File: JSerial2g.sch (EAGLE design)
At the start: 59 parts, among them CN1 USBMOLEX, IC1 FT232RL, Q1 2N3904SOT23, Q2 2N3904SOT23, Q3 BC547, Q4 BC547, X1 RJ45-8X

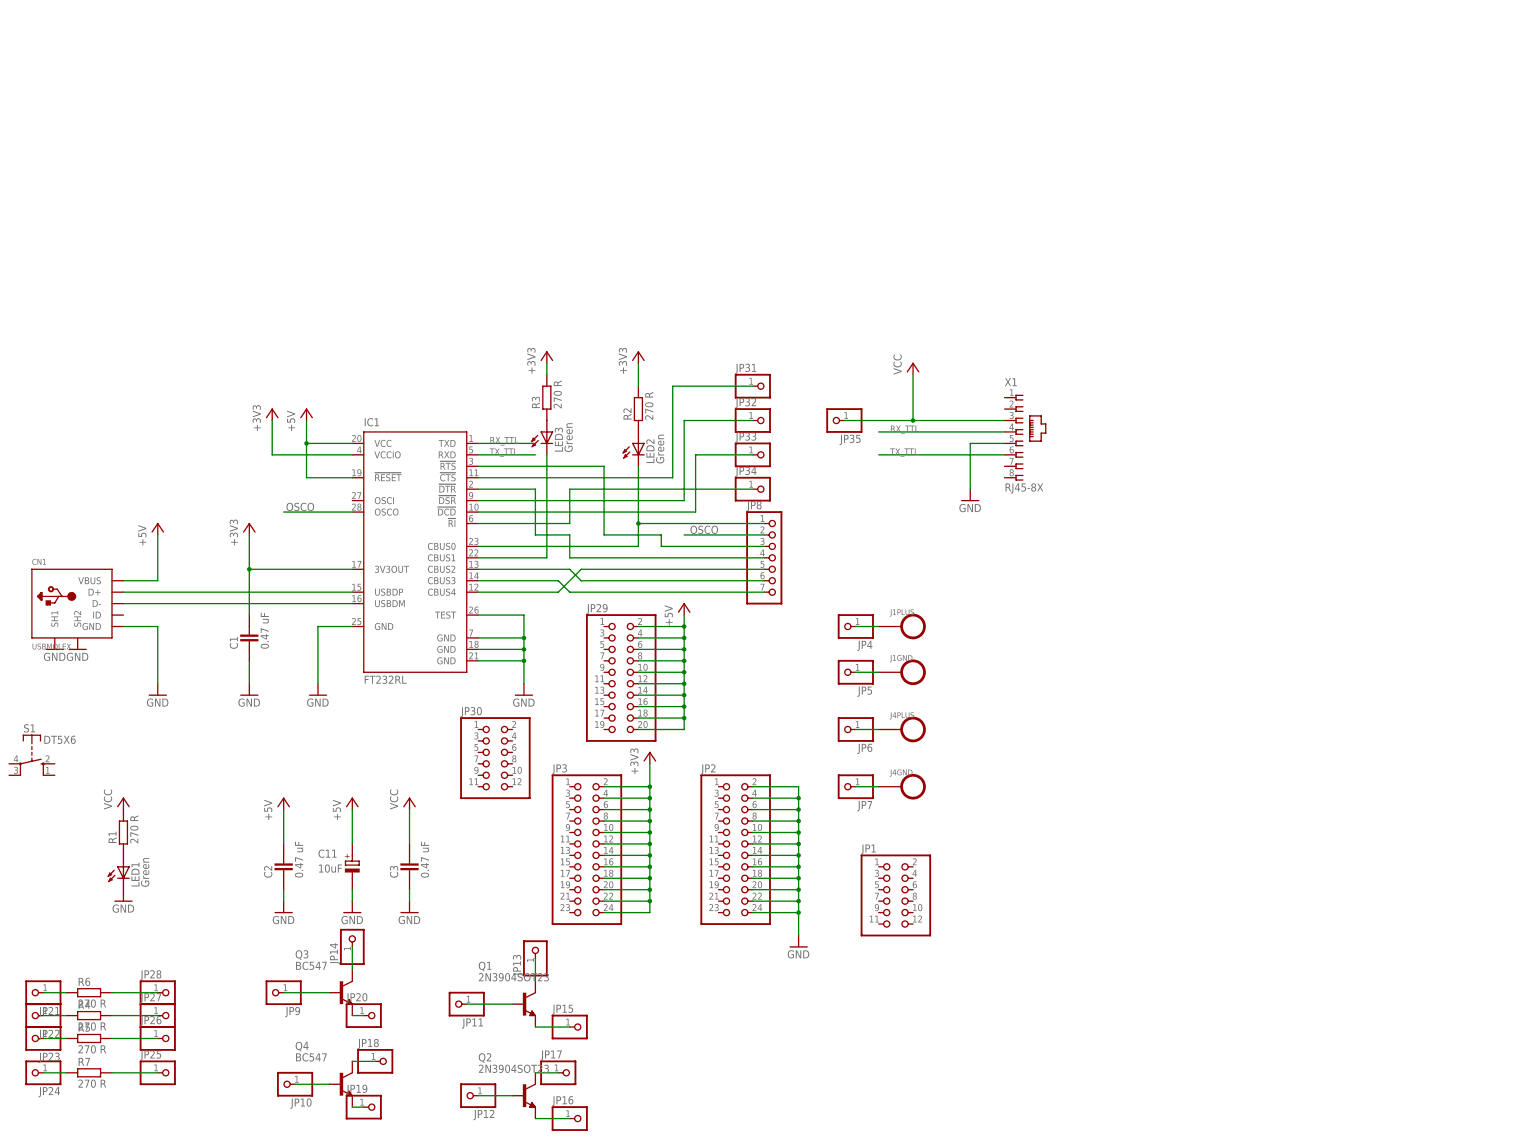
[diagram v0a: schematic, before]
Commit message: JSerial 2G in progress
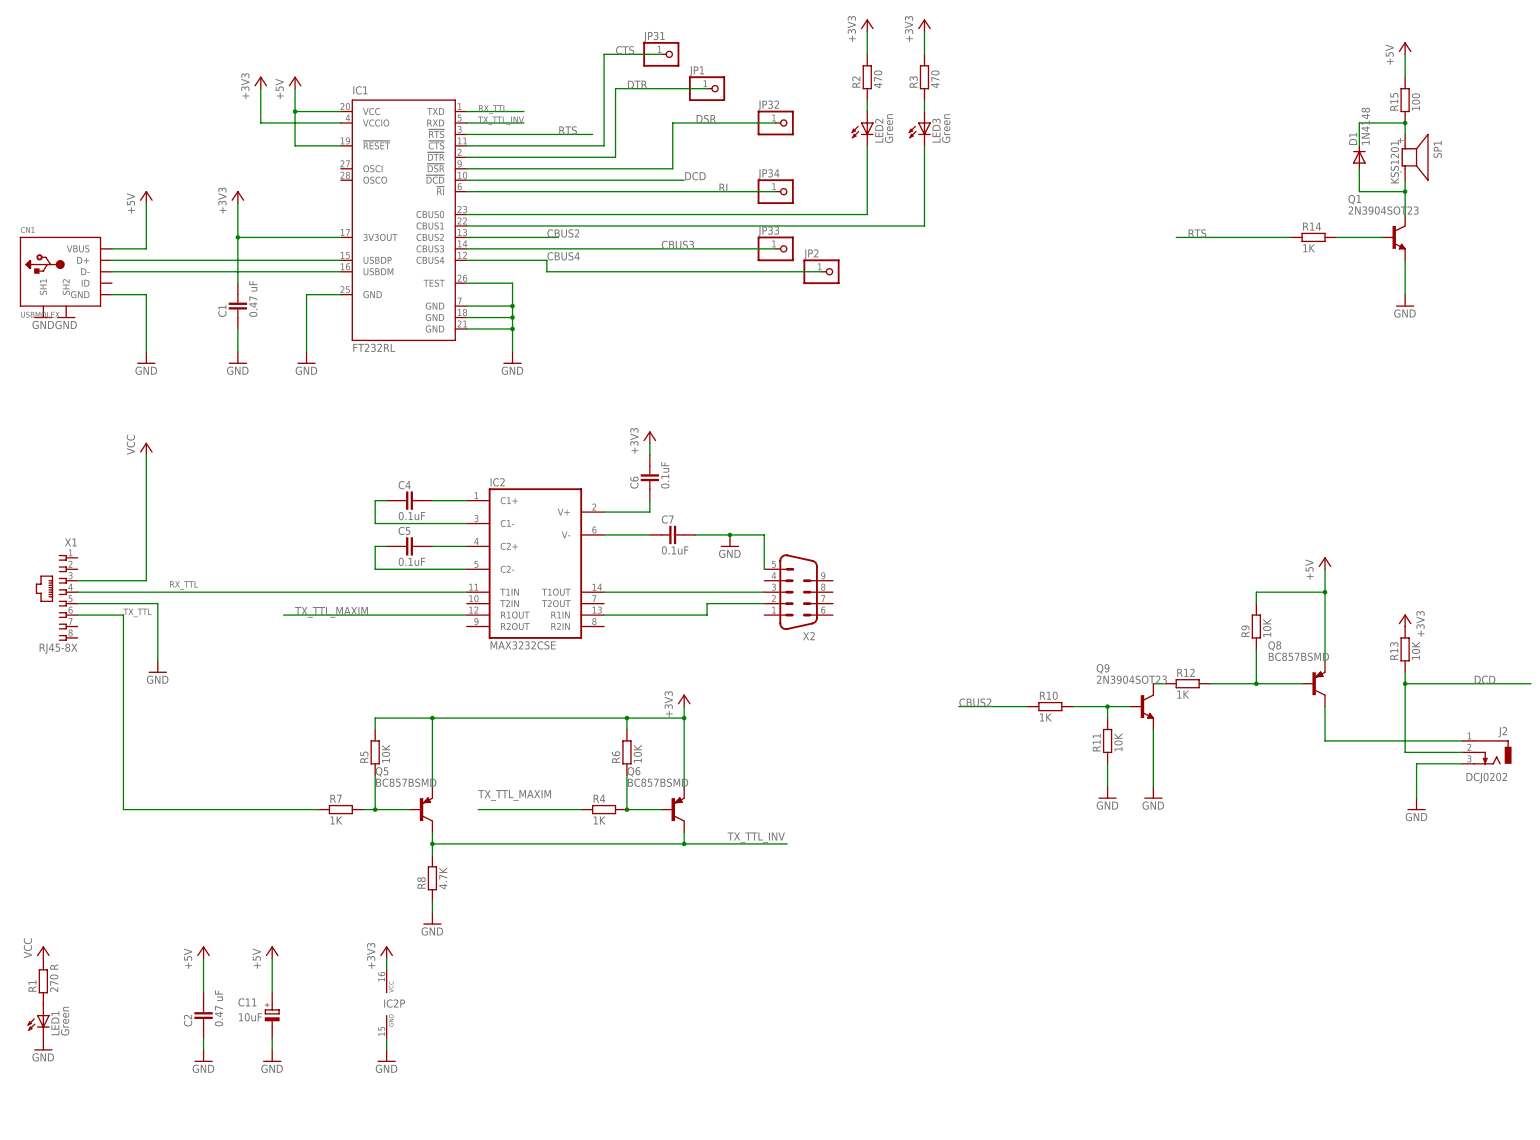
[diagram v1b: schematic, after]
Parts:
- removed C3: 0.47 uF, ipc-7351-capacitor:CAPACITOR_0805
- removed J1, J4: (no value), jlab:POWER-OUT
- removed JP10, JP11, JP12, JP13, JP14, JP15, JP16, JP17, JP18, JP19, JP20, JP21, JP22, JP23, JP24, JP25, JP26, JP27, JP28, JP35, JP4, JP5, JP6, JP7, JP9: (no value), pinhead:PINHD-1X1
- removed JP29: (no value), pinhead:PINHD-2X10
- removed JP3: (no value), pinhead:PINHD-2X12
- removed JP30: (no value), pinhead:PINHD-2X6
- removed JP8: (no value), pinhead:PINHD-1X7
- removed Q2: 2N3904SOT23, transistor-npn:2N3904SOT23
- removed Q3, Q4: BC547, transistor-npn:BC547
- removed S1: DT5X6, jlab:DT5X6
- added C4, C5, C6, C7: 0.1uF, ipc-7351-capacitor:CAPACITOR_0805
- added D1: 1N4148, diode:DIODE-SOD123
- added IC2: MAX3232CSE, maxim:MAX3232CSE
- added J2: DCJ0202, con-jack:DCJ0202
- added Q5, Q6, Q8: BC857BSMD, transistor-pnp:BC857BSMD
- added Q9: 2N3904SOT23, transistor-npn:2N3904SOT23
- added R10, R12, R14: 1K, ipc-7351-resistor:RESISTOR_0805
- added R11, R13, R9: 10K, ipc-7351-resistor:RESISTOR_0805
- added R15: 100, ipc-7351-resistor:RESISTOR_0805
- added R8: 4.7K, ipc-7351-resistor:RESISTOR_0805
- added SP1: KSS1201, buzzer:KSS1201
- added X2: (no value), jlab:M09D
- JP1: device pinhead:PINHD-2X6 -> pinhead:PINHD-1X1
- JP2: device pinhead:PINHD-2X12 -> pinhead:PINHD-1X1
- LED2, LED3: device jlab:LEDCHIP-LED0805 -> jlab:LED3MM
- R2, R3: value 270 R -> 470
- R4, R7: value 270 R -> 1K
- R5, R6: value 270 R -> 10K
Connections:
- net RT renamed RI
- removed net N$23: JP22.1, R4.1
- removed net N$24: JP14.1, Q3.C
- removed net N$25: JP18.1, Q4.C
- removed net N$26: JP19.1, Q4.E
- removed net N$27: JP20.1, Q3.E
- removed net N$28: JP23.1, R5.1
- removed net N$29: JP24.1, R7.1
- removed net N$30: JP13.1, Q1.C
- removed net N$31: JP15.1, Q1.E
- removed net N$32: JP17.1, Q2.C
- removed net N$33: JP16.1, Q2.E
- removed net N$34: JP25.1, R7.2
- removed net N$35: JP26.1, R5.2
- removed net N$36: JP27.1, R4.2
- removed net N$37: JP28.1, R6.2
- removed net OSCO: IC1.OSCO, JP8.2
- new net N$13: IC2G$1.R1IN, X2.2
- new net N$14: J2.1, Q8.C
- new net N$15: Q5.B, R5.1, R7.2
- new net N$16: Q6.B, R4.2, R6.1
- new net N$17: Q9.B, R10.2, R11.2
- new net N$2: C4.1, IC2G$1.C1-
- new net N$7: C4.2, IC2G$1.C1+
- new net N$8: C5.1, IC2G$1.C2-
- new net TX_TTL_INV: IC1.RXD, Q5.C, Q6.C, R8.2
- new net TX_TTL_MAXIM: IC2G$1.R1OUT, R4.1
- net +3V3: now also C6.2, IC2P.VCC, Q5.E, Q6.E, R13.2, R5.2, R6.2; no longer JP3.10, JP3.12, JP3.14, JP3.16, JP3.18, JP3.2, JP3.20, JP3.22, JP3.24, JP3.4, JP3.6, JP3.8
- net +5V: now also Q8.E, R15.2, R9.2; no longer JP29.10, JP29.12, JP29.14, JP29.16, JP29.18, JP29.2, JP29.20, JP29.4, JP29.6, JP29.8
- net CBUS0: no longer JP8.1
- net CBUS2: now also R10.1; no longer JP8.6
- net CBUS3: now also JP33.1; no longer JP8.7
- net CBUS4: now also JP2.1; no longer JP8.5
- net DCD: now also J2.2, R13.1; no longer JP33.1
- net DTR: now also JP1.1; no longer JP8.4
- net GND: now also C7.2, IC2P.GND, J2.3, Q1.E, Q9.E, R11.1, R8.1, X2.5; no longer C3.1, JP2.10, JP2.12, JP2.14, JP2.16, JP2.18, JP2.2, JP2.20, JP2.22, JP2.24, JP2.4, JP2.6, JP2.8
- net N$10: now also C6.1, IC2G$1.V+; no longer J1GND.P$1, JP5.1
- net N$11: now also C7.1, IC2G$1.V-; no longer J4PLUS.P$1, JP6.1
- net N$12: now also IC2G$1.T1OUT, X2.3; no longer J4GND.P$1, JP7.1
- net N$18: now also Q9.C, R12.1; no longer JP9.1, Q3.B
- net N$19: now also Q8.B, R12.2, R9.1; no longer JP10.1, Q4.B
- net N$20: now also Q1.B, R14.2; no longer JP12.1, Q2.B
- net N$21: now also D1.A, Q1.C, SP1.2; no longer JP11.1, Q1.B
- net N$22: now also D1.C, R15.1, SP1.1; no longer JP21.1, R6.1
- net N$9: now also C5.2, IC2G$1.C2+; no longer J1PLUS.P$1, JP4.1
- net RTS: now also R14.1; no longer JP8.3
- net RX_TTL: now also IC2G$1.T1IN
- net TX_TTL: now also R7.1; no longer IC1.RXD
- net VCC: no longer C3.2, JP35.1
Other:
- moved on the sheet: C1, C11, C2, CN1, IC1, JP31, JP32, JP33, JP34, LED1, LED2, LED3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
